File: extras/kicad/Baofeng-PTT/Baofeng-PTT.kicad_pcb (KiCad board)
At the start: 2 copper layers, 58.4 x 30.5 mm, 10 parts, among them J1 AI, J2 AO, J4 PTT, J8 Baofeng, U1 ULN2003

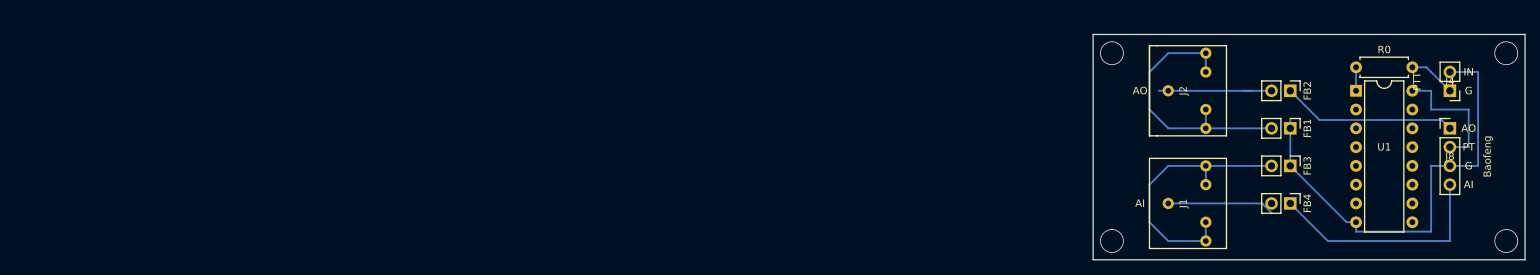
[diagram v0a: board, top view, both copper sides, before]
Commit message: Cleanup Kikad project
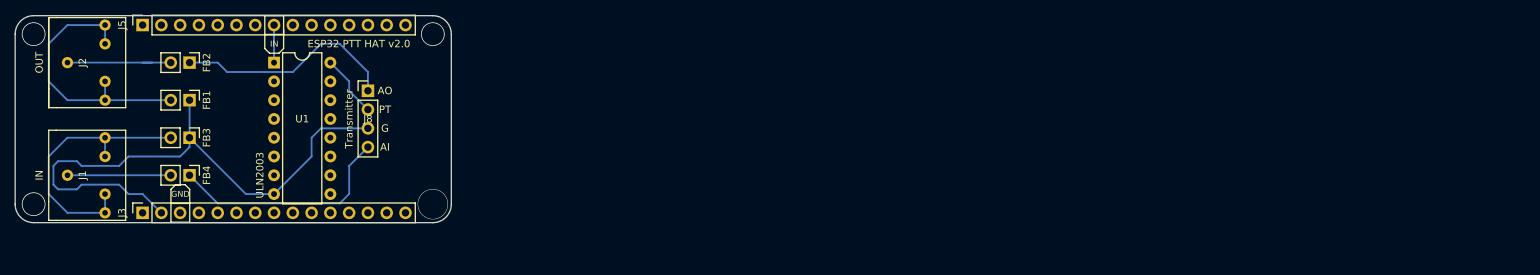
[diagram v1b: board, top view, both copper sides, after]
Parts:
- removed J4: PTT, Connector_PinHeader_2.54mm:PinHeader_1x02_P2.54mm_Vertical
- removed R0: R0, Resistor_THT:R_Axial_DIN0207_L6.3mm_D2.5mm_P7.62mm_Horizontal
- added J3: Conn_01x15, Connector_PinSocket_2.54mm:PinSocket_1x15_P2.54mm_Vertical, F.Cu at (36.5, 44.5)
- added J5: Esp32, Connector_PinSocket_2.54mm:PinSocket_1x15_P2.54mm_Vertical, F.Cu at (36.5, 19.1)
- J1: value AI -> IN
- J2: value AO -> OUT
- J8: value Baofeng -> Transmitter
- moved FB1 148.9 mm to (42.9, 29.2)
- moved FB2 148.9 mm to (42.9, 24.1)
- moved FB3 148.9 mm to (42.9, 34.3)
- moved FB4 148.9 mm to (42.9, 39.4)
- moved J1 148.9 mm to (28.9, 39.4)
- moved J2 148.9 mm to (28.9, 24.1)
- moved J8 146.4 mm to (67.0, 27.9)
- moved U1 146.4 mm to (54.3, 24.1)
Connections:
- U1 pad 1: Net-(R0-Pad1) -> D25
- U1 pad 10: Net-(U1-Pad10) -> (no net)
- U1 pad 11: Net-(U1-Pad11) -> (no net)
- U1 pad 12: Net-(U1-Pad12) -> (no net)
- U1 pad 13: Net-(U1-Pad13) -> (no net)
- U1 pad 14: Net-(U1-Pad14) -> (no net)
- U1 pad 15: Net-(U1-Pad15) -> (no net)
- U1 pad 2: Net-(U1-Pad2) -> (no net)
- U1 pad 3: Net-(U1-Pad3) -> (no net)
- U1 pad 4: Net-(U1-Pad4) -> (no net)
- U1 pad 5: Net-(U1-Pad5) -> (no net)
- U1 pad 6: Net-(U1-Pad6) -> (no net)
- U1 pad 7: Net-(U1-Pad7) -> (no net)
- U1 pad 9: Net-(U1-Pad9) -> (no net)
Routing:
- net GND: track 61.6 -> 78.0 mm
- net PT: track 17.8 -> 8.45 mm
- net AO: track 23.7 -> 31.6 mm
- net D25: track 0.00 -> 7.62 mm
- net Net-(J4-Pad1): track 6.40 -> 0.00 mm
- net Net-(R0-Pad1): track 2.54 -> 0.00 mm
- net Net-(FB2-Pad2): track 16.5 -> 15.2 mm
- net Net-(FB4-Pad2): track 14.5 -> 14.0 mm
- net Net-(FB3-Pad2): vias 0 -> 1
- net Net-(FB1-Pad2): vias 0 -> 1
- net (no net): vias 4 -> 2
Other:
- board size 58.4 x 30.5 mm -> 59 x 28 mm
- board text added: "ESP32 PTT HAT v2.0"
- board text added: "GND"
